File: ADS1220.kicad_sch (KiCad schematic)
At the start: 4 parts, among them U4 ADS1232IPW

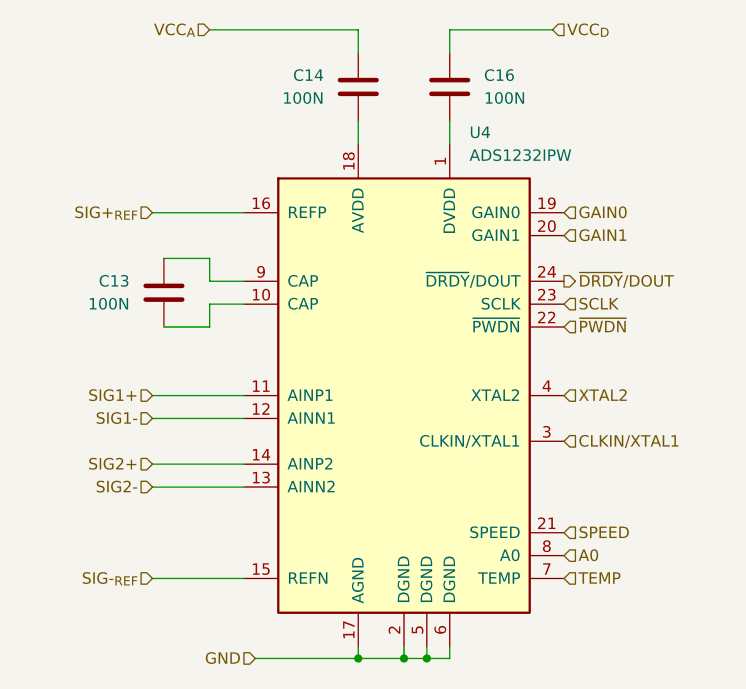
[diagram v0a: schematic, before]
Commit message: loadcell parts
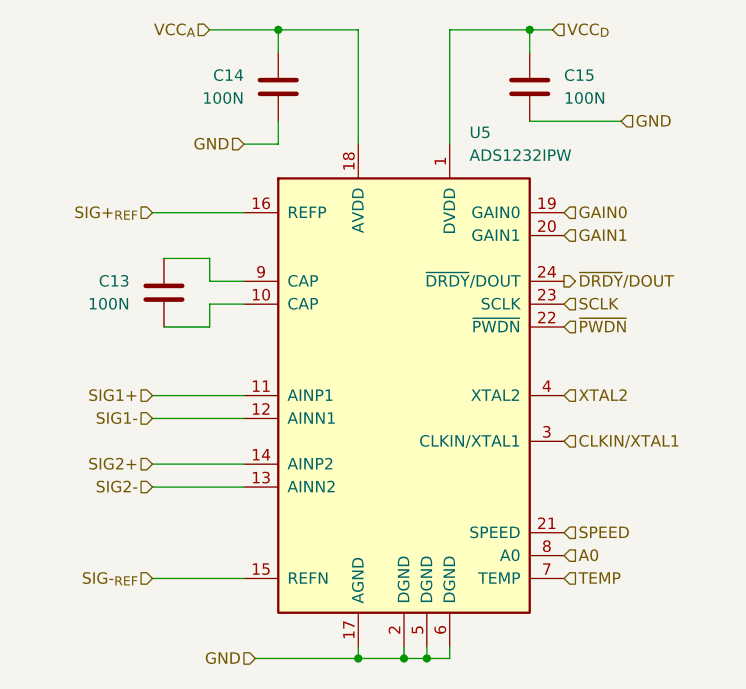
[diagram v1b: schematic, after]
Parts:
- removed U4: ADS1232IPW, symbol Analog_ADC:ADS1232IPW
- added U5: ADS1232IPW, Package_SO:TSSOP-24_4.4x7.8mm_P0.65mm, symbol william_adc:ADS1232IPW
- renumbered C16 to C15
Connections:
- net A0: now also U5.8 (A0)
- net CLKIN/XTAL1: now also U5.3 (CLKIN/XTAL1)
- net GAIN0: now also U5.19 (GAIN0)
- net GAIN1: now also U5.20 (GAIN1)
- net GND: now also C14.2, C15.2, U5.17 (AGND), U5.2 (DGND), U5.5 (DGND), U5.6 (DGND)
- net SCLK: now also U5.23 (SCLK)
- net SIG+_{REF}: now also U5.16 (REFP)
- net SIG-_{REF}: now also U5.15 (REFN)
- net SIG1+: now also U5.11 (AINP1)
- net SIG1-: now also U5.12 (AINN1)
- net SIG2+: now also U5.14 (AINP2)
- net SIG2-: now also U5.13 (AINN2)
- net SPEED: now also U5.21 (SPEED)
- net TEMP: now also U5.7 (TEMP)
- net VCC_{A}: now also U5.18 (AVDD)
- net VCC_{D}: now also U5.1 (DVDD)
- net XTAL2: now also U5.4 (XTAL2)
- net ~{DRDY}/DOUT: now also U5.24 (~{DRDY}/DOUT)
- net ~{PWDN}: now also U5.22 (~{PWDN})
- net at C13.1: now also U5.9 (CAP)
- net at C13.2: now also U5.10 (CAP)
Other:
- moved on the sheet: C14, C15
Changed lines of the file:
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@@
   (junction (at 154.94 128.27) (diameter 0) (color 0 0 0 0)
   )
+  (junction (at 166.37 58.42) (diameter 0) (color 0 0 0 0)
+  )
+  (junction (at 138.43 58.42) (diameter 0) (color 0 0 0 0)
+  )
   (junction (at 147.32 128.27) (diameter 0) (color 0 0 0 0)
   )
@@
     (stroke (width 0) (type default))
   )
+  (wire (pts (xy 166.37 68.58) (xy 176.53 68.58))
+    (stroke (width 0) (type default))
+  )
   (wire (pts (xy 152.4 127) (xy 152.4 128.27))
     (stroke (width 0) (type default))
@@
     (stroke (width 0) (type default))
   )
+  (wire (pts (xy 166.37 58.42) (xy 166.37 60.96))
+    (stroke (width 0) (type default))
+  )
   (wire (pts (xy 157.48 128.27) (xy 157.48 127))
     (stroke (width 0) (type default))
   )
-  (wire (pts (xy 130.81 58.42) (xy 147.32 58.42))
+  (wire (pts (xy 138.43 71.12) (xy 138.43 68.58))
+    (stroke (width 0) (type default))
+  )
+  (wire (pts (xy 134.62 71.12) (xy 138.43 71.12))
+    (stroke (width 0) (type default))
+  )
+  (wire (pts (xy 130.81 58.42) (xy 138.43 58.42))
     (stroke (width 0) (type default))
   )
@@
     (stroke (width 0) (type default))
   )
-  (wire (pts (xy 147.32 58.42) (xy 147.32 60.96))
-    (stroke (width 0) (type default))
-  )
-  (wire (pts (xy 147.32 68.58) (xy 147.32 71.12))
-    (stroke (width 0) (type default))
-  )
-  (wire (pts (xy 157.48 68.58) (xy 157.48 71.12))
+  (wire (pts (xy 147.32 58.42) (xy 147.32 71.12))
+    (stroke (width 0) (type default))
+  )
+  (wire (pts (xy 166.37 58.42) (xy 157.48 58.42))
     (stroke (width 0) (type default))
   )
@@
     (stroke (width 0) (type default))
   )
-  (wire (pts (xy 168.91 58.42) (xy 157.48 58.42))
+  (wire (pts (xy 168.91 58.42) (xy 166.37 58.42))
+    (stroke (width 0) (type default))
+  )
+  (wire (pts (xy 138.43 58.42) (xy 138.43 60.96))
     (stroke (width 0) (type default))
   )
@@
     (stroke (width 0) (type default))
   )
+  (wire (pts (xy 138.43 58.42) (xy 147.32 58.42))
+    (stroke (width 0) (type default))
+  )
   (wire (pts (xy 130.81 83.82) (xy 130.81 86.36))
     (stroke (width 0) (type default))
@@
     (stroke (width 0) (type default))
   )
-  (wire (pts (xy 157.48 58.42) (xy 157.48 60.96))
-    (stroke (width 0) (type default))
+  (wire (pts (xy 157.48 58.42) (xy 157.48 71.12))
+    (stroke (width 0) (type default))
+  )
+  (hierarchical_label "GND" (shape input) (at 134.62 71.12 180) (fields_autoplaced)
+    (effects (font (size 1.27 1.27)) (justify right))
   )
   (hierarchical_label "VCC_{A}" (shape input) (at 130.81 58.42 180) (fields_autoplaced)
@@
     (effects (font (size 1.27 1.27)) (justify right))
   )
+  (hierarchical_label "GND" (shape input) (at 176.53 68.58 0) (fields_autoplaced)
+    (effects (font (size 1.27 1.27)) (justify left))
+  )
   (hierarchical_label "SIG2-" (shape input) (at 124.46 109.22 180) (fields_autoplaced)
     (effects (font (size 1.27 1.27)) (justify right))
@@
     (effects (font (size 1.27 1.27)) (justify right))
   )
-  (symbol (lib_id "Device:C") (at 147.32 64.77 0) (mirror y) (unit 1)
-    (in_bom yes) (on_board yes) (dnp no)
-    (property "Reference" "C14" (at 143.51 63.5 0)
-      (effects (font (size 1.27 1.27)) (justify left))
-    )
-    (property "Value" "100N" (at 143.51 66.04 0)
-      (effects (font (size 1.27 1.27)) (justify left))
-    )
-    (property "Footprint" "Capacitor_SMD:C_0603_1608Metric" (at 146.3548 68.58 0)
-      (effects (font (size 1.27 1.27)) hide)
-    )
-    (property "Datasheet" "~" (at 147.32 64.77 0)
-      (effects (font (size 1.27 1.27)) hide)
-    )
-    (pin "1")
-    (pin "2")
-    (instances
-      (project "main"
-        (path "/6bf28e97-b749-4534-8a2e-432f9a4b1c9e/0fcaa597-73a2-400e-99ba-2fcca2977ff3/29b4d57a-b37e-4bc9-9adb-d6acc2b22778/dc6d7d4b-2f06-4d39-8328-e356fb7157af"
-          (reference "C14") (unit 1)
-        )
-      )
-    )
-  )
-  (symbol (lib_id "Device:C") (at 125.73 87.63 0) (mirror y) (unit 1)
-    (in_bom yes) (on_board yes) (dnp no)
-    (property "Reference" "C13" (at 121.92 86.36 0)
-      (effects (font (size 1.27 1.27)) (justify left))
-    )
-    (property "Value" "100N" (at 121.92 88.9 0)
-      (effects (font (size 1.27 1.27)) (justify left))
-    )
-    (property "Footprint" "Capacitor_SMD:C_0603_1608Metric" (at 124.7648 91.44 0)
-      (effects (font (size 1.27 1.27)) hide)
-    )
-    (property "Datasheet" "~" (at 125.73 87.63 0)
-      (effects (font (size 1.27 1.27)) hide)
-    )
-    (pin "1")
-    (pin "2")
-    (instances
-      (project "main"
-        (path "/6bf28e97-b749-4534-8a2e-432f9a4b1c9e/0fcaa597-73a2-400e-99ba-2fcca2977ff3/29b4d57a-b37e-4bc9-9adb-d6acc2b22778/dc6d7d4b-2f06-4d39-8328-e356fb7157af"
-          (reference "C13") (unit 1)
-        )
-      )
-    )
-  )
-  (symbol (lib_id "Analog_ADC:ADS1232IPW") (at 152.4 99.06 0) (unit 1)
+  (symbol (lib_id "william_adc:ADS1232IPW") (at 152.4 99.06 0) (unit 1)
     (in_bom yes) (on_board yes) (dnp no) (fields_autoplaced)
-    (property "Reference" "U4" (at 159.6741 69.85 0)
+    (property "Reference" "U5" (at 159.6741 69.85 0)
       (effects (font (size 1.27 1.27)) (justify left))
     )
@@
       (effects (font (size 1.27 1.27)) (justify left))
     )
-    (property "Footprint" "" (at 152.4 99.06 0)
+    (property "Footprint" "Package_SO:TSSOP-24_4.4x7.8mm_P0.65mm" (at 152.4 99.06 0)
       (effects (font (size 1.27 1.27) italic) hide)
     )
@@
       (project "main"
         (path "/6bf28e97-b749-4534-8a2e-432f9a4b1c9e/0fcaa597-73a2-400e-99ba-2fcca2977ff3/29b4d57a-b37e-4bc9-9adb-d6acc2b22778/dc6d7d4b-2f06-4d39-8328-e356fb7157af"
-          (reference "U4") (unit 1)
+          (reference "U5") (unit 1)
         )
       )
     )
   )
-  (symbol (lib_id "Device:C") (at 157.48 64.77 0) (unit 1)
+  (symbol (lib_id "Device:C") (at 138.43 64.77 0) (mirror y) (unit 1)
     (in_bom yes) (on_board yes) (dnp no)
-    (property "Reference" "C16" (at 161.29 63.5 0)
-      (effects (font (size 1.27 1.27)) (justify left))
-    )
-    (property "Value" "100N" (at 161.29 66.04 0)
-      (effects (font (size 1.27 1.27)) (justify left))
-    )
-    (property "Footprint" "Capacitor_SMD:C_0603_1608Metric" (at 158.4452 68.58 0)
-      (effects (font (size 1.27 1.27)) hide)
-    )
-    (property "Datasheet" "~" (at 157.48 64.77 0)
-      (effects (font (size 1.27 1.27)) hide)
-    )
+    (property "Reference" "C14" (at 134.62 63.5 0)
+      (effects (font (size 1.27 1.27)) (justify left))
+    )
+    (property "Value" "100N" (at 134.62 66.04 0)
+      (effects (font (size 1.27 1.27)) (justify left))
+    )
+    (property "Footprint" "Capacitor_SMD:C_0603_1608Metric" (at 137.4648 68.58 0)
+      (effects (font (size 1.27 1.27)) hide)
+    )
+    (property "Datasheet" "~" (at 138.43 64.77 0)
+      (effects (font (size 1.27 1.27)) hide)
+    )
+    (pin "1")
+    (pin "2")
+    (instances
+      (project "main"
+        (path "/6bf28e97-b749-4534-8a2e-432f9a4b1c9e/0fcaa597-73a2-400e-99ba-2fcca2977ff3/29b4d57a-b37e-4bc9-9adb-d6acc2b22778/dc6d7d4b-2f06-4d39-8328-e356fb7157af"
+          (reference "C14") (unit 1)
+        )
+      )
+    )
+  )
+  (symbol (lib_id "Device:C") (at 125.73 87.63 0) (mirror y) (unit 1)
+    (in_bom yes) (on_board yes) (dnp no)
+    (property "Reference" "C13" (at 121.92 86.36 0)
+      (effects (font (size 1.27 1.27)) (justify left))
+    )
+    (property "Value" "100N" (at 121.92 88.9 0)
+      (effects (font (size 1.27 1.27)) (justify left))
+    )
+    (property "Footprint" "Capacitor_SMD:C_0603_1608Metric" (at 124.7648 91.44 0)
+      (effects (font (size 1.27 1.27)) hide)
+    )
+    (property "Datasheet" "~" (at 125.73 87.63 0)
+      (effects (font (size 1.27 1.27)) hide)
+    )
+    (pin "1")
+    (pin "2")
+    (instances
+      (project "main"
+        (path "/6bf28e97-b749-4534-8a2e-432f9a4b1c9e/0fcaa597-73a2-400e-99ba-2fcca2977ff3/29b4d57a-b37e-4bc9-9adb-d6acc2b22778/dc6d7d4b-2f06-4d39-8328-e356fb7157af"
+          (reference "C13") (unit 1)
+        )
+      )
+    )
+  )
+  (symbol (lib_id "Device:C") (at 166.37 64.77 0) (unit 1)
+    (in_bom yes) (on_board yes) (dnp no)
+    (property "Reference" "C15" (at 170.18 63.5 0)
+      (effects (font (size 1.27 1.27)) (justify left))
+    )
+    (property "Value" "100N" (at 170.18 66.04 0)
+      (effects (font (size 1.27 1.27)) (justify left))
+    )
+    (property "Footprint" "Capacitor_SMD:C_0603_1608Metric" (at 167.3352 68.58 0)
+      (effects (font (size 1.27 1.27)) hide)
+    )
+    (property "Datasheet" "~" (at 166.37 64.77 0)
+      (effects (font (size 1.27 1.27)) hide)
+    )
